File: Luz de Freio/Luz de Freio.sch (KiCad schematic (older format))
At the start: 54 parts, among them J1 Screw_Terminal_01x02, J2 Screw_Terminal_01x02, K1 RELAY_19.1x15.5mm, Q1 BC548, Q2 IRF3205, U1 MC34063AP, U2 TL431DBZ, U3 LM358

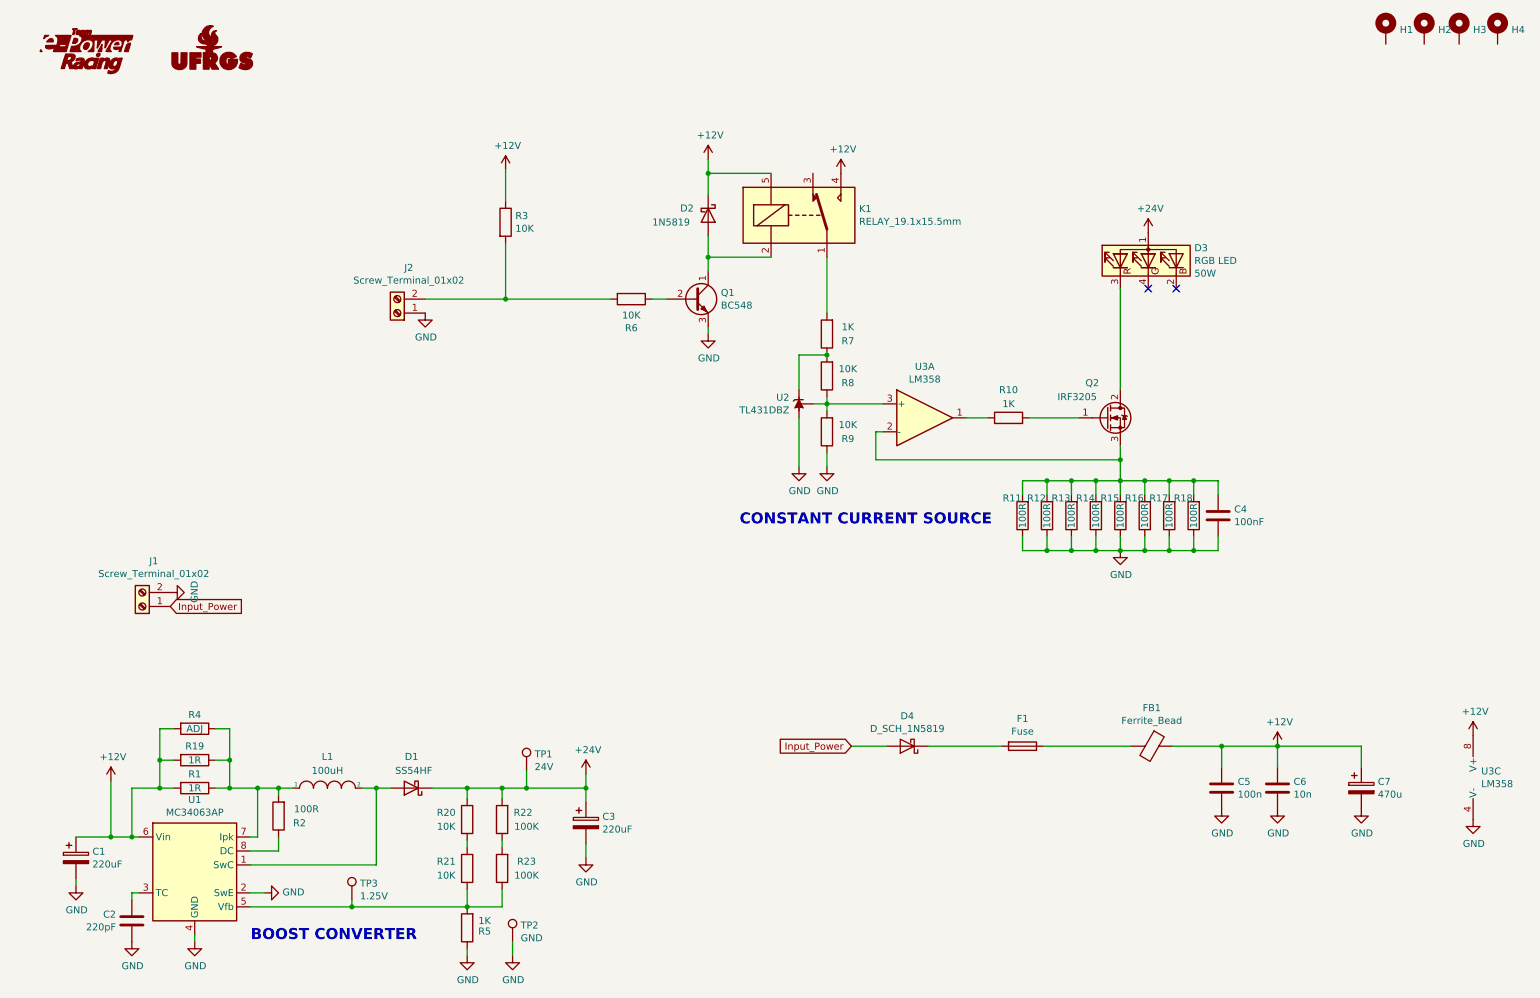
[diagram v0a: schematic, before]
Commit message: Fixed Schematic and Layout
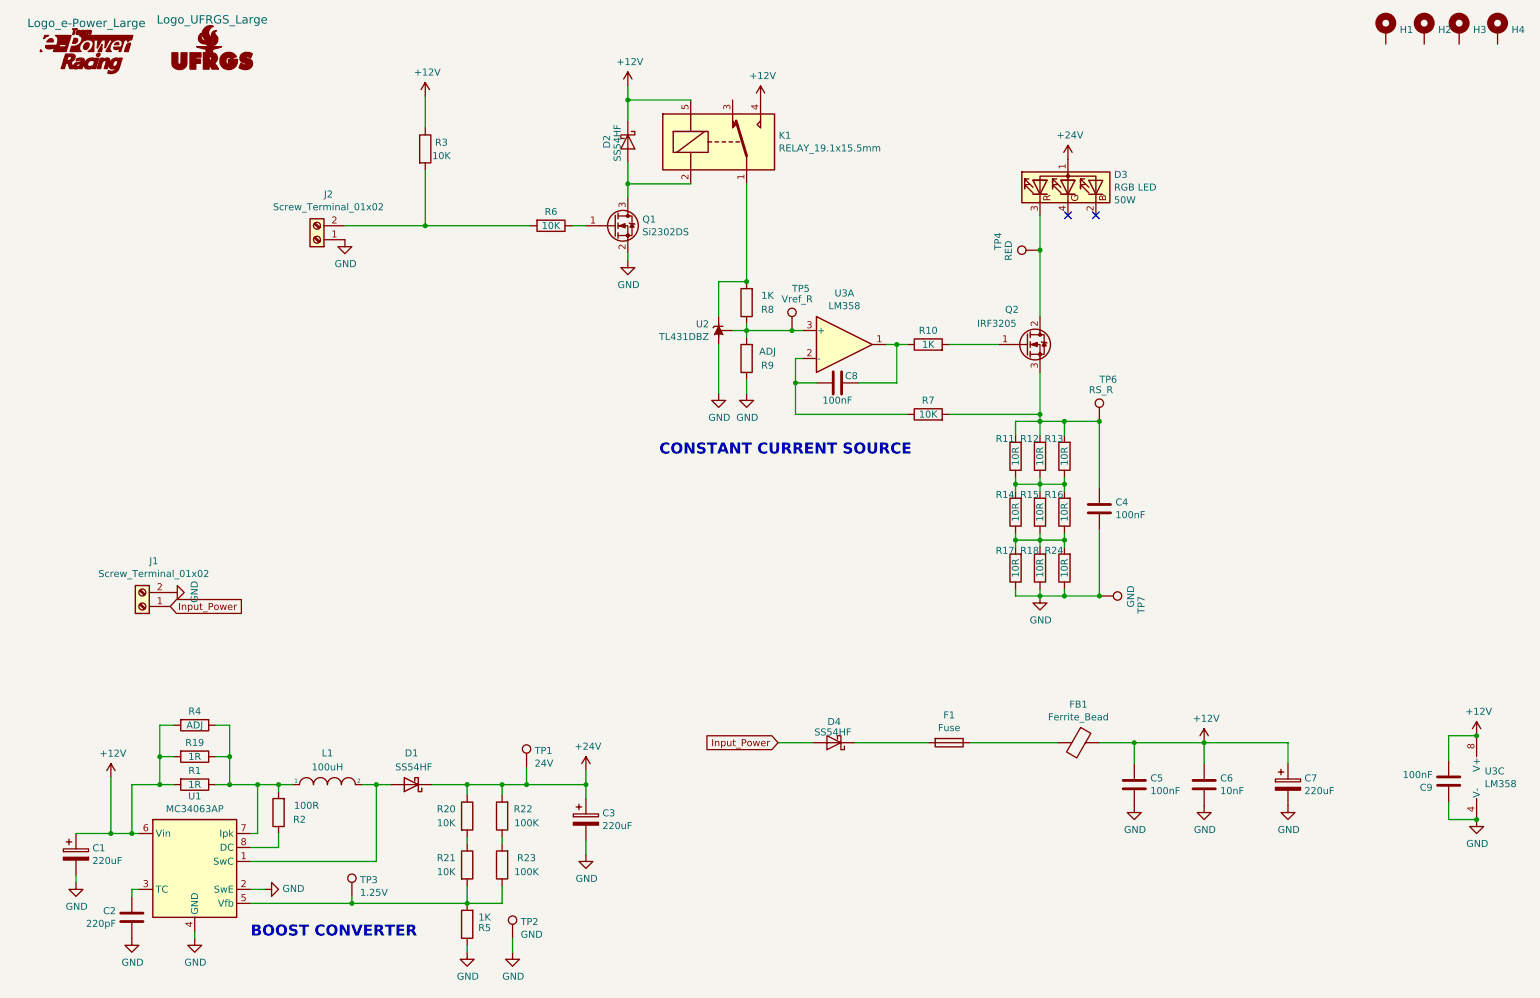
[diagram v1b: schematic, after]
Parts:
- removed D2: 1N5819, e-Power:DO-214AC, symbol Diode:1N5819
- removed D4: D_SCH_1N5819, e-Power:DO-214AC, symbol e-Power:D_SCH_1N5819
- removed Q1: BC548, Package_TO_SOT_SMD:SOT-23, symbol Transistor_BJT:BC548
- added C8: 100nF, Capacitor_SMD:C_0805_2012Metric, symbol Device:C
- added C9: 100nF, Capacitor_SMD:C_0805_2012Metric_Pad1.15x1.40mm_HandSolder, symbol Device:C
- added D2, D4: SS54HF, e-Power:DO-214AC, symbol e-Power:SS54HF
- added Q1: Si2302DS, Package_TO_SOT_SMD:SOT-23, symbol e-Power:Si2302DS
- added R24: 10R, Resistor_SMD:R_0805_2012Metric_Pad1.15x1.40mm_HandSolder, symbol Device:R
- added TP4: RED, e-Power:TestPoint_Pad_D1.0mm, symbol Connector:TestPoint
- added TP5: Vref_R, e-Power:TestPoint_Pad_D1.0mm, symbol Connector:TestPoint
- added TP6: RS_R, e-Power:TestPoint_Pad_D1.0mm, symbol Connector:TestPoint
- added TP7: GND, e-Power:TestPoint_Pad_D1.0mm, symbol Connector:TestPoint
- C5: value 100n -> 100nF
- C6: value 10n -> 10nF
- C7: value 470u -> 220uF
- D3, J1, J2: footprint e-Power:TerminalBlock_Phoenix_MKDS-1,5-2_1x02_P5.08mm_Horizontal_3D -> e-Power:TerminalBlock_Phoenix_MKDS-1,5-2_1x02_P5.08mm_Horizontal
- FB1: footprint e-Power:FB_0603_1608Metric -> e-Power:FB_0805_2012Metric
- L1: footprint e-Power:L_10.4x10.4_H4.8 -> e-Power:L_12x12mm_H6mm
- R11, R12, R13, R14, R15, R16, R17, R18: value 100R -> 10R
- R7: value 1K -> 10K
- R8: value 10K -> 1K
- R9: value 10K -> ADJ
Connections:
- net +12V: now also C9.1, D2.1 (K)
- net GND: now also C9.2, Q1.2 (S), R24.1, TP7.1; no longer R11.1, R12.1, R13.1, R14.1, R15.1, R16.1
- net Input_Power: now also D4.2 (A)
- net at K1.2: now also D2.2 (A), Q1.3 (D)
- net at R6.1: now also Q1.1 (G)
- net at D3.3 (RK), Q2.2 (D): now also TP4.1
- net at R8.1, R9.2, U2.2 (REF)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: now also TP5.1
- net at R8.2, U2.1 (K): now also K1.1; no longer R7.1
- net at R10.1, U3.1: now also C8.1
- net at R7.2: now also C4.2, Q2.3 (S), R11.2, R12.2, R13.2, TP6.1; no longer K1.1
- net at F1.2: now also D4.1 (K)
- new net: C8.2, R7.1, U3.2 (-)
- new net: R14.1, R15.1, R16.1, R17.2, R18.2, R24.2
- new net: R11.1, R12.1, R13.1, R14.2, R15.2, R16.2
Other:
- moved on the sheet: C1, C2, C3, C4, C5, C6, C7, D1, D3, F1, FB1, J2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
